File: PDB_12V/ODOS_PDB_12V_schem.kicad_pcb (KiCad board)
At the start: 2 copper layers, 30 x 42 mm, 8 parts, among them J1 XT30UPB-F, J2 XT30UPB-F, J3 XT30UPB-F, J4 XT30UPB-F, J5 XT30UPB-F, J6 XT30UPB-F

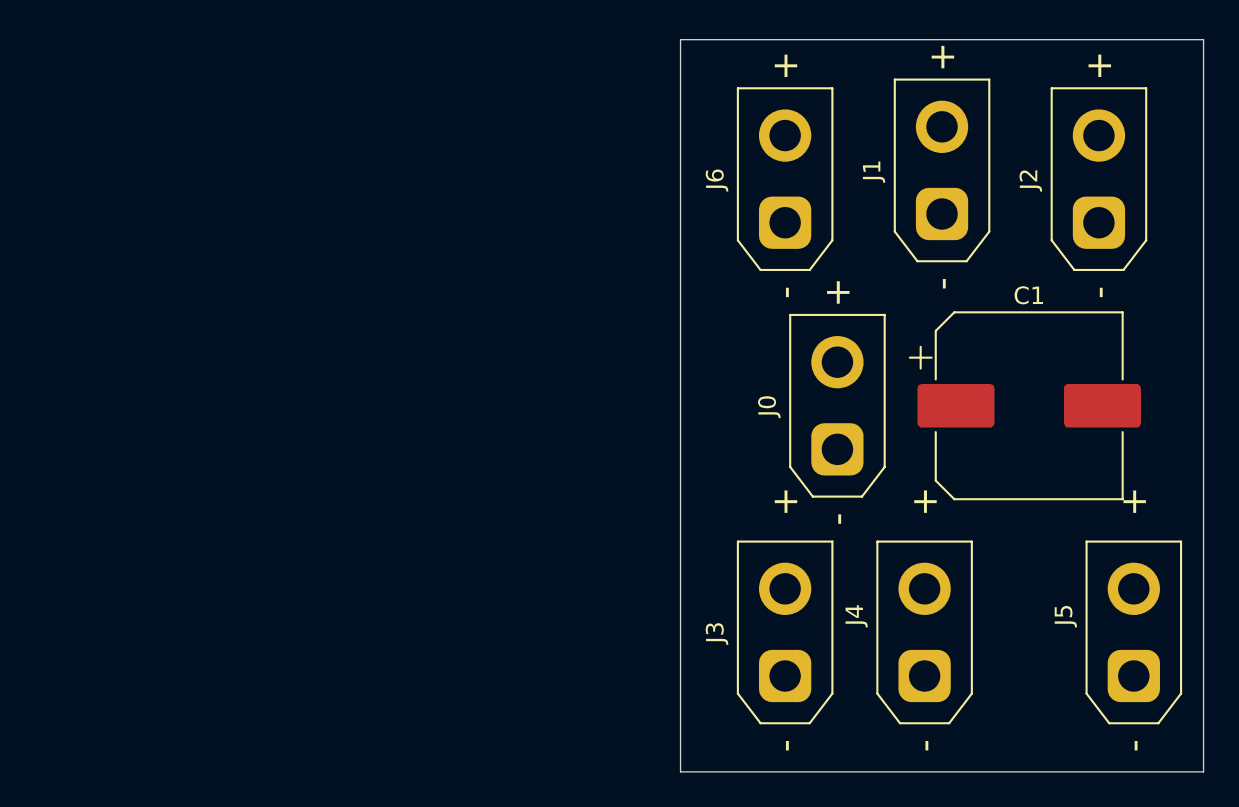
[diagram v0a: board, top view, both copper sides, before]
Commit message: nouveau layout et 2 plans pour gnd et +12
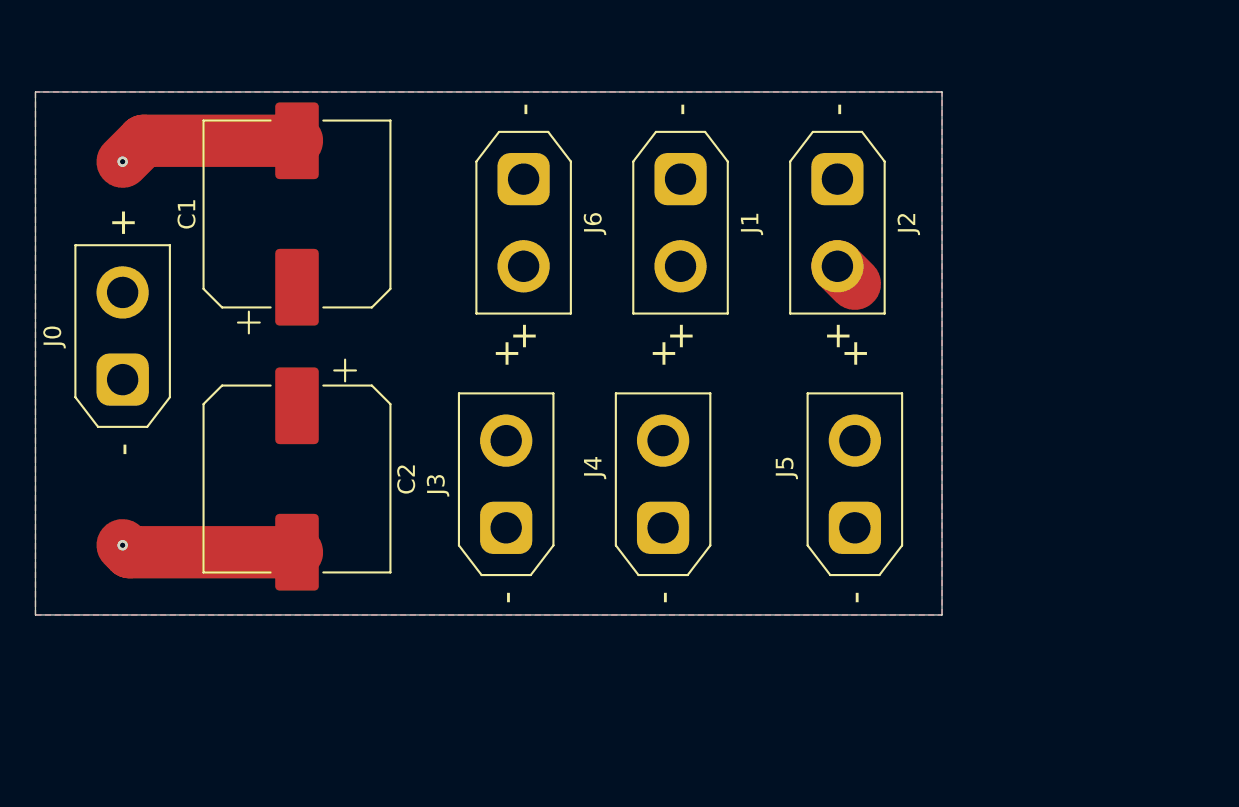
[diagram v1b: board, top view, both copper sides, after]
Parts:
- added C2: 820µF, Capacitor_SMD:CP_Elec_10x10.5, F.Cu at (122.0, 84.2)
- moved C1 43.4 mm to (122.0, 69.0), turned to 90 degrees
- moved J0 41.2 mm to (112.0, 78.5)
- moved J3 18.1 mm to (134.0, 87.0)
- moved J5 18.1 mm to (154.0, 87.0)
- moved J4 17.2 mm to (143.0, 87.0)
- moved J2 15.2 mm to (153.0, 67.0), turned to -90 degrees
- moved J6 15.2 mm to (135.0, 67.0), turned to -90 degrees
- moved J1 15.1 mm to (144.0, 67.0), turned to -90 degrees
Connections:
- J1 pad 1: +12V -> GND
- J1 pad 2: GND -> +12V
- J2 pad 1: +12V -> GND
- J2 pad 2: GND -> +12V
- J3 pad 1: +12V -> GND
- J3 pad 2: GND -> +12V
- J4 pad 1: +12V -> GND
- J4 pad 2: GND -> +12V
- J5 pad 1: +12V -> GND
- J5 pad 2: GND -> +12V
- J6 pad 1: +12V -> GND
- J6 pad 2: GND -> +12V
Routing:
- net GND: track 0.00 -> 20.7 mm, vias 0 -> 2
- net +12V: track 0.00 -> 1.41 mm
- added copper zone on F.Cu, net +12V
- added copper zone on B.Cu, net GND
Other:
- board size 30 x 42 mm -> 52 x 30 mm
